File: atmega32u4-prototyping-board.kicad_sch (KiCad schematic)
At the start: 18 parts, among them J1 USB_C_Receptacle_USB2.0_16P, J2 Conn_01x16, J3 Conn_01x16, U1 ATmega32U4-M, Y1 CSTNE16M0V53C000R0

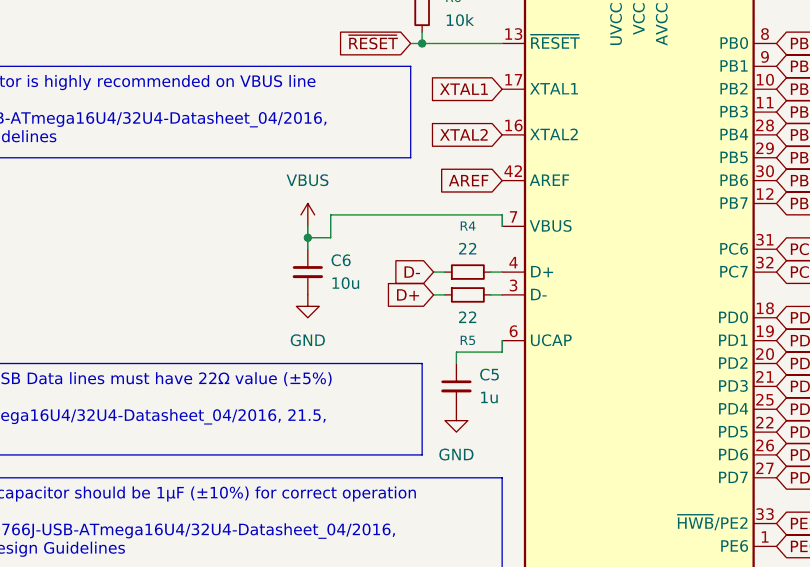
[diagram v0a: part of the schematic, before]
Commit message: Update board image
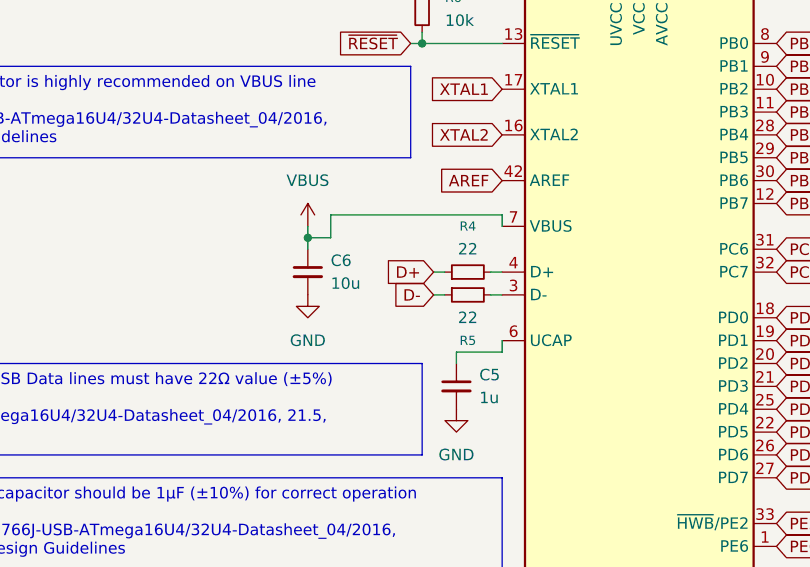
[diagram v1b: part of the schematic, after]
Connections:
- net D+: now also R4.1; no longer R5.1
- net D-: now also R5.1; no longer R4.1
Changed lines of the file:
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@@
+		)
+	)
+	(global_label "D-"
+		(shape input)
+		(at 40.64 80.01 180)
+		(fields_autoplaced yes)
+		(effects
+			(font
+				(size 1.27 1.27)
+			)
+			(justify right)
+		)
+		(property "Intersheetrefs" "${INTERSHEET_REFS}"
+			(at 34.8124 80.01 0)
+			(effects
+				(font
+					(size 1.27 1.27)
+				)
+				(justify right)
+				(hide yes)
+			)
 		)
 	)
@@
 	(global_label "D+"
 		(shape input)
-		(at 40.64 80.01 180)
-		(fields_autoplaced yes)
-		(effects
-			(font
-				(size 1.27 1.27)
-			)
-			(justify right)
-		)
-		(property "Intersheetrefs" "${INTERSHEET_REFS}"
-			(at 34.8124 80.01 0)
-			(effects
-				(font
-					(size 1.27 1.27)
-				)
-				(justify right)
-				(hide yes)
-			)
-		)
-	)
-	(global_label "D-"
-		(shape input)
 		(at 40.64 77.47 180)
